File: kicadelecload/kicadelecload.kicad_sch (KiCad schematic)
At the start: 28 parts, among them Q1 IRF540N, Q2 IRF540N, Q3 IRF540N, Q4 IRF540N, Q5 IRF540N, U1 ESP32-S2-DEVKITC-1, U2 LM358, U3 TL431D

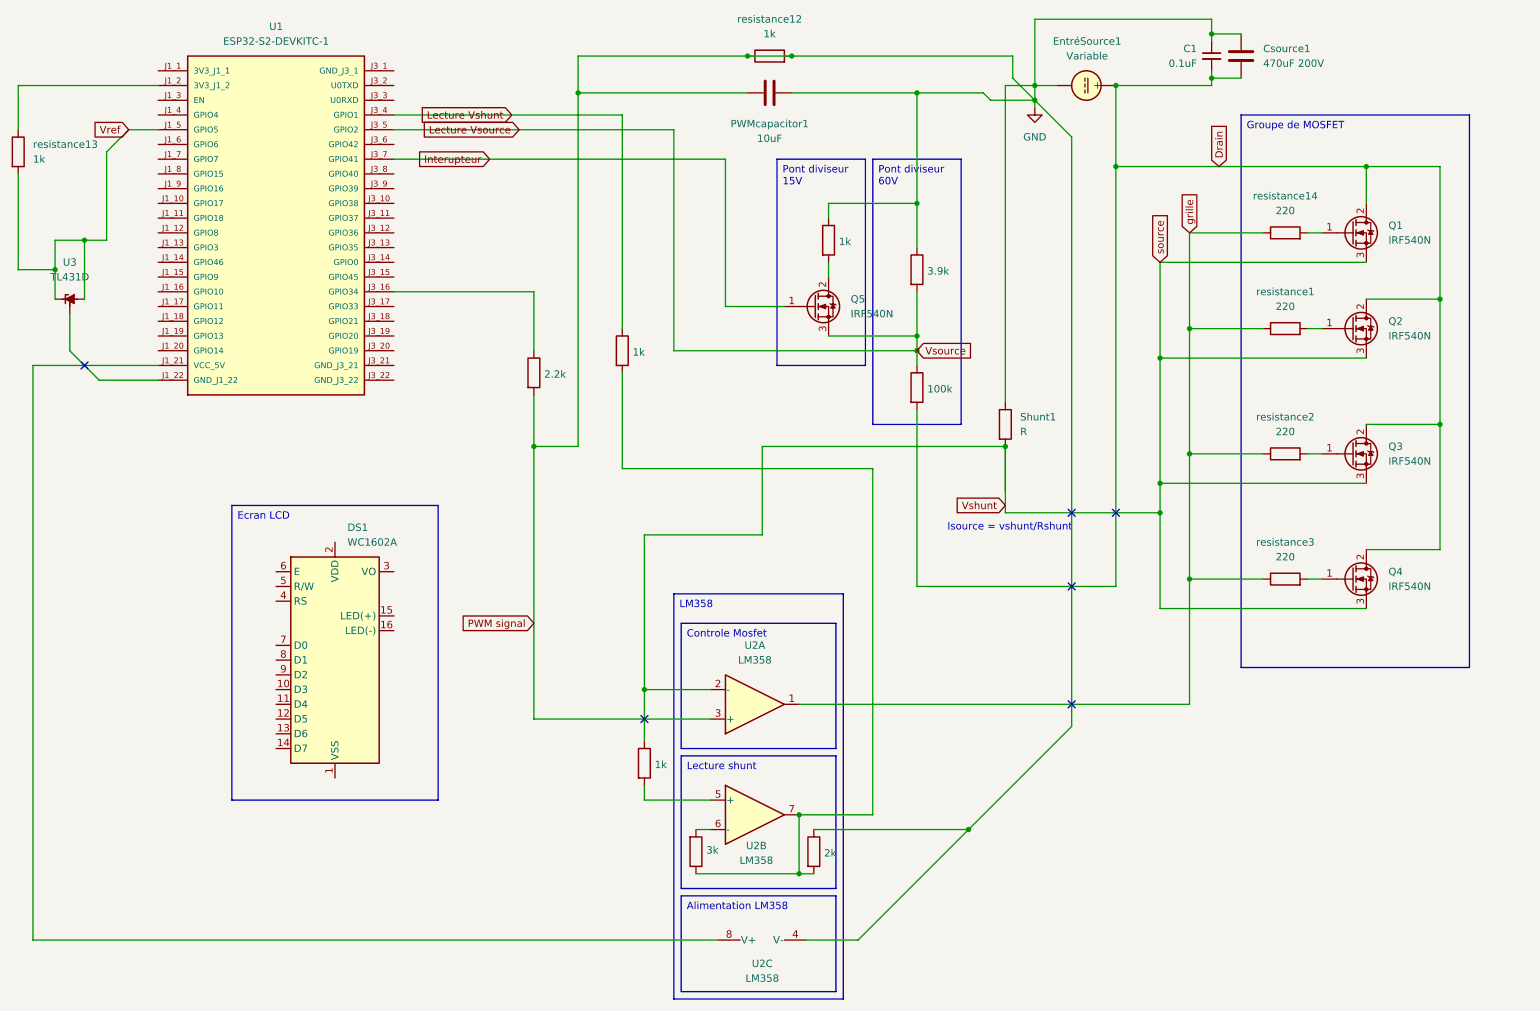
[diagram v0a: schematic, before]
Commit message: schema electrique V1 commit 4
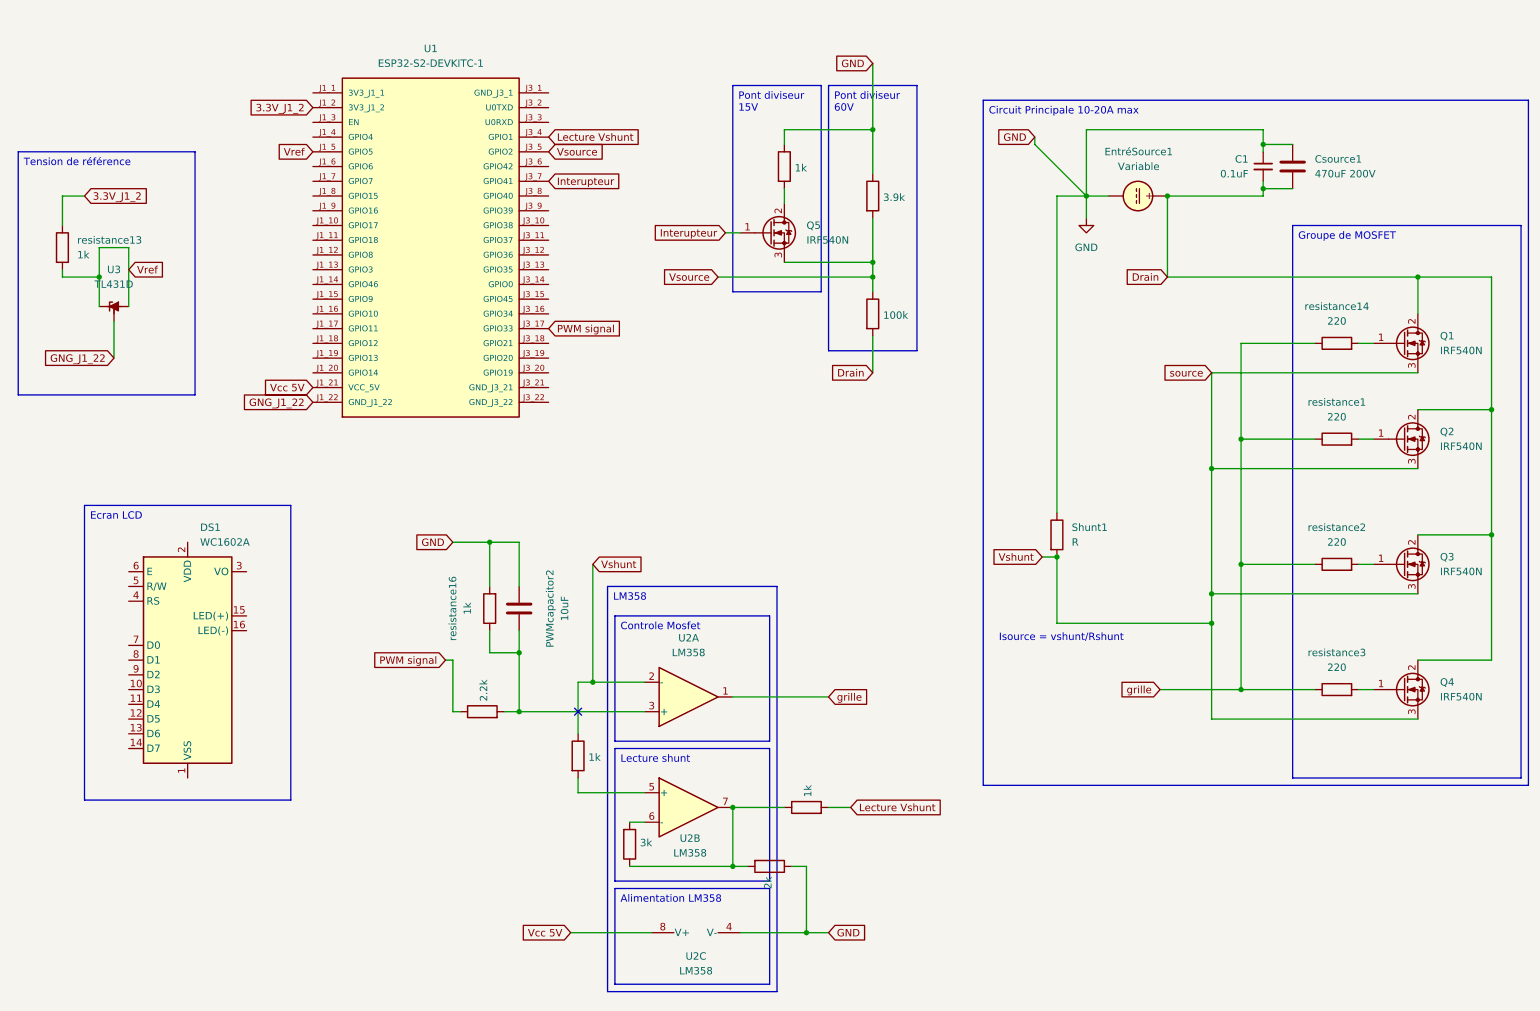
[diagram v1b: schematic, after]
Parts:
- removed PWMcapacitor1: 10uF, symbol Device:C
- removed resistance10, resistance12: 1k, symbol Device:R
- added PWMcapacitor2: 10uF, symbol Device:C
- added resistance15: 2.2k, symbol Device:R
- added resistance16: 1k, symbol Device:R
- resistance11: value 2.2k -> 1k
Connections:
- net GND: now also PWMcapacitor2.2, resistance16.2; no longer U2.3 (+), resistance11.2
- net Lecture Vshunt: now also resistance11.2
- net at resistance11.1: now also U2.7, resistance8.1, resistance9.2; no longer U1.J3_16 (GPIO34)
- net 3.3V_J1_2: now reaches U1.J1_2 (3V3_J1_2), resistance13.1
- net GNG_J1_22: now reaches U1.J1_22 (GND_J1_22), U3.8 (REF)
- net Vcc 5V: now reaches U1.J1_21 (VCC_5V), U2.8 (V+)
- net PWM signal: now reaches U1.J3_17 (GPIO33)
- net PWM signal: now also resistance15.1
- net Lecture Vsource renamed Vsource
- new net: PWMcapacitor2.1, U2.3 (+), resistance15.2, resistance16.1
- no-connect marks 6 -> 1
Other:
- moved on the sheet: C1, Csource1, DS1, EntréSource1, Q1, Q2, Q3, Q4, Q5, Shunt1, U1, U2A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
